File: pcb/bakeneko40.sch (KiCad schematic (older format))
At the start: 15 parts

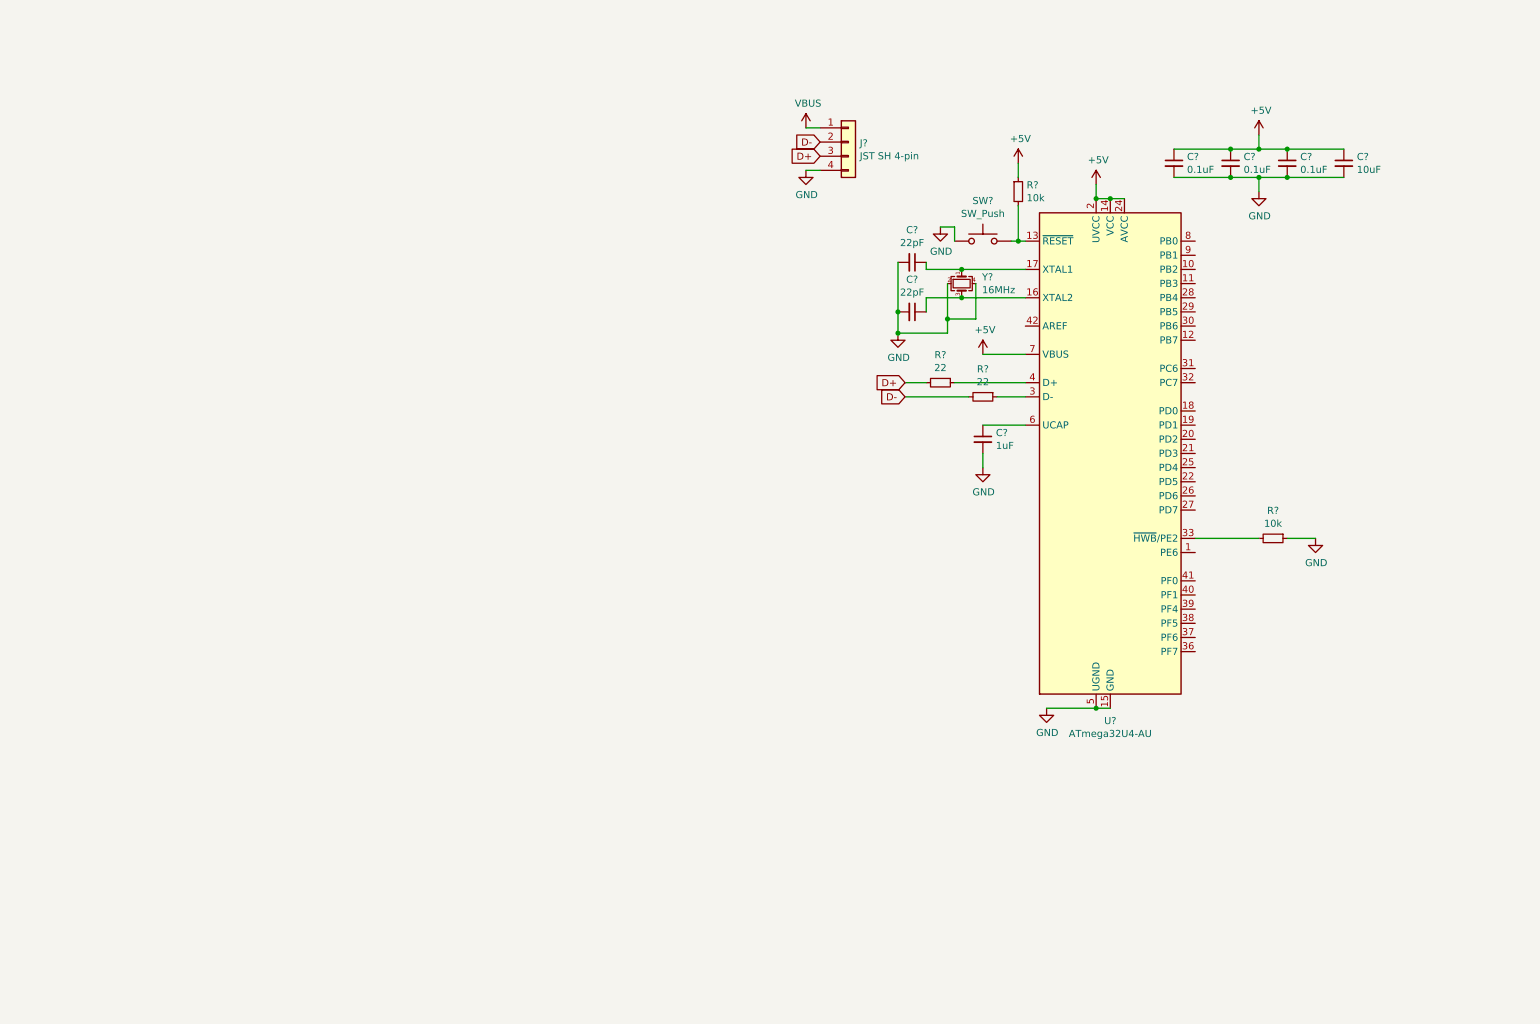
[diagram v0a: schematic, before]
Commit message: sch updates
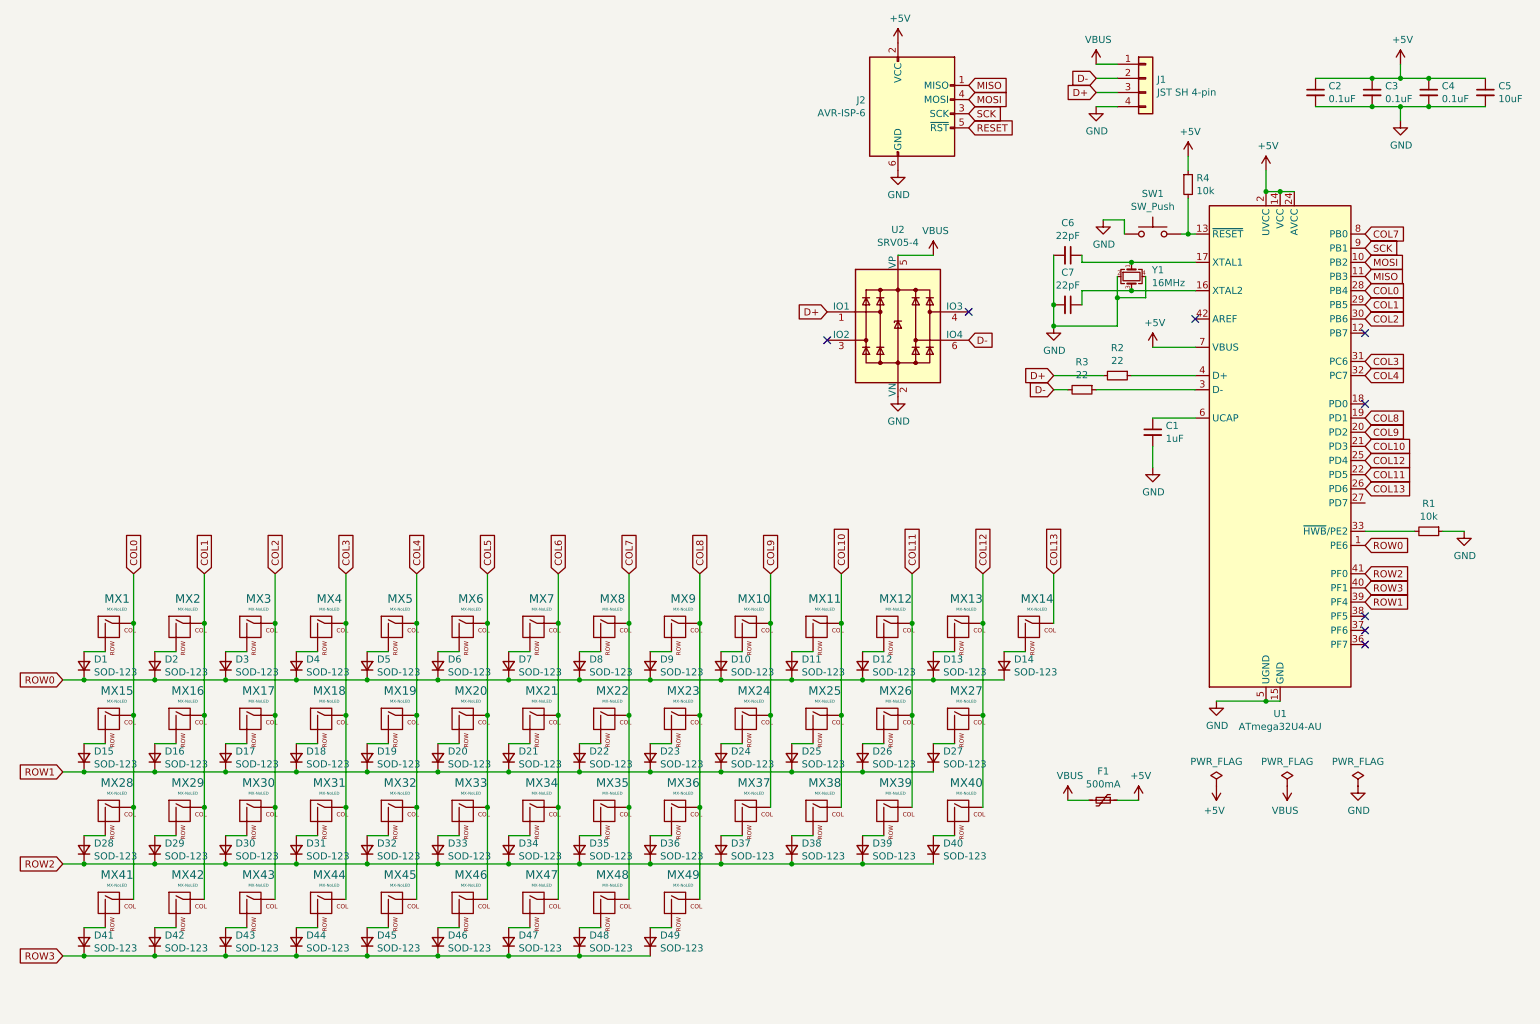
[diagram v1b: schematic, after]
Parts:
- removed C?: 1uF, symbol Device:C_Small
- removed C? (x3): 0.1uF, symbol Device:C_Small
- removed C?: 10uF, symbol Device:C_Small
- removed C? (x2): 22pF, symbol Device:C_Small
- removed J?: JST SH 4-pin, Connector_JST:JST_SH_SM04B-SRSS-TB_1x04-1MP_P1.00mm_Horizontal, symbol Connector_Generic:Conn_01x04
- removed R? (x2): 10k, symbol Device:R_Small
- removed R? (x2): 22, symbol Device:R_Small
- removed SW?: SW_Push, symbol Switch:SW_Push
- removed U?: ATmega32U4-AU, Package_QFP:TQFP-44_10x10mm_P0.8mm, symbol MCU_Microchip_ATmega:ATmega32U4-AU
- removed Y?: 16MHz, symbol Device:Crystal_GND24_Small
- added C1: 1uF, Capacitor_SMD:C_0805_2012Metric, symbol Device:C_Small
- added C2, C3, C4: 0.1uF, Capacitor_SMD:C_0805_2012Metric, symbol Device:C_Small
- added C5: 10uF, Capacitor_SMD:C_0805_2012Metric, symbol Device:C_Small
- added C6: 22pF, Capacitor_SMD:C_0805_2012Metric, symbol Device:C_Small
- added C7: 22pF, Diode_SMD:D_SOD-123, symbol Device:C_Small
- added D1, D10, D11, D12, D13, D14, D15, D16, D17, D18, D19, D2, D20, D21, D22, D23, D24, D25, D26, D27, D28, D29, D3, D30, D31, D32, D33, D34, D35, D36, D37, D38, D39, D4, D40, D41, D42, D43, D44, D45, D46, D47, D48, D49, D5, D6, D7, D8, D9: SOD-123, Diode_SMD:D_SOD-123, symbol Device:D_Small
- added F1: 500mA, Fuse:Fuse_1206_3216Metric, symbol Device:Polyfuse_Small
- added J1: JST SH 4-pin, random-keyboard-parts:JST-SR-4, symbol Connector_Generic:Conn_01x04
- added J2: AVR-ISP-6, random-keyboard-parts:Reset_Pretty-Mask, symbol Connector:AVR-ISP-6
- added MX1, MX10, MX11, MX12, MX13, MX14, MX16, MX17, MX18, MX19, MX2, MX20, MX21, MX22, MX23, MX24, MX25, MX26, MX29, MX3, MX30, MX31, MX32, MX33, MX34, MX35, MX36, MX37, MX38, MX4, MX40, MX49, MX5, MX6, MX7, MX8, MX9: MX-NoLED, MX_Only:MXOnly-1U-NoLED, symbol MX_Alps_Hybrid:MX-NoLED
- added MX15, MX39, MX41, MX43, MX46, MX48: MX-NoLED, MX_Only:MXOnly-1.25U-NoLED, symbol MX_Alps_Hybrid:MX-NoLED
- added MX27, MX28: MX-NoLED, MX_Only:MXOnly-1.75U-NoLED, symbol MX_Alps_Hybrid:MX-NoLED
- added MX42, MX47: MX-NoLED, MX_Only:MXOnly-1.5U-NoLED, symbol MX_Alps_Hybrid:MX-NoLED
- added MX44: MX-NoLED, MX_Only:MXOnly-2.25U-NoLED, symbol MX_Alps_Hybrid:MX-NoLED
- added MX45: MX-NoLED, MX_Only:MXOnly-2.75U-NoLED, symbol MX_Alps_Hybrid:MX-NoLED
- added R1, R4: 10k, Resistor_SMD:R_0805_2012Metric, symbol Device:R_Small
- added R2, R3: 22, Resistor_SMD:R_0805_2012Metric, symbol Device:R_Small
- added SW1: SW_Push, random-keyboard-parts:SKQG-1155865, symbol Switch:SW_Push
- added U1: ATmega32U4-AU, Package_QFP:TQFP-44_10x10mm_P0.8mm, symbol MCU_Microchip_ATmega:ATmega32U4-AU
- added U2: SRV05-4, Package_TO_SOT_SMD:SOT-23-6, symbol Power_Protection:SRV05-4
- added Y1: 16MHz, Crystal:Crystal_SMD_3225-4Pin_3.2x2.5mm, symbol Device:Crystal_GND24_Small
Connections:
- net +5V: now also C2.1, C3.1, C4.1, C5.1, F1.1, J2.2 (VCC), R4.1, U1.14 (VCC), U1.2 (UVCC), U1.24 (AVCC), U1.34 (VCC), U1.44 (AVCC), U1.7 (VBUS)
- net D+: now also J1.3 (Pin_3), R2.2, U2.1 (IO1)
- net D-: now also J1.2 (Pin_2), R3.2, U2.6 (IO4)
- net GND: now also C1.2, C2.2, C3.2, C4.2, C5.2, C6.2, C7.2, J1.4 (Pin_4), J2.6 (GND), R1.1, SW1.1, U1.15 (GND), U1.23 (GND), U1.35 (GND), U1.43 (GND), U1.5 (UGND), U2.2 (VN), Y1.2, Y1.4
- net VBUS: now also F1.2, J1.1 (Pin_1), U2.5 (VP)
- new net: R2.1, U1.4 (D+)
- new net: R3.1, U1.3 (D-)
- new net: C1.1, U1.6 (UCAP)
- new net: C6.1, U1.17 (XTAL1), Y1.1
- new net: C7.1, U1.16 (XTAL2), Y1.3
- new net: R4.2, SW1.2, U1.13 (~RESET)
- new net: D1.2 (A), MX1.2 (ROW)
- new net: D2.2 (A), MX2.2 (ROW)
- new net: D3.2 (A), MX3.2 (ROW)
- new net: D4.2 (A), MX4.2 (ROW)
- new net: D5.2 (A), MX5.2 (ROW)
- new net: D6.2 (A), MX6.2 (ROW)
- new net: D7.2 (A), MX7.2 (ROW)
- new net: D8.2 (A), MX8.2 (ROW)
- new net: D9.2 (A), MX9.2 (ROW)
- new net: D10.2 (A), MX10.2 (ROW)
- new net: D11.2 (A), MX11.2 (ROW)
- new net: D12.2 (A), MX12.2 (ROW)
- new net: D13.2 (A), MX13.2 (ROW)
- new net: D14.2 (A), MX14.2 (ROW)
- new net: D15.2 (A), MX15.2 (ROW)
- new net: D16.2 (A), MX16.2 (ROW)
- new net: D17.2 (A), MX17.2 (ROW)
- new net: D18.2 (A), MX18.2 (ROW)
- new net: D19.2 (A), MX19.2 (ROW)
- new net: D20.2 (A), MX20.2 (ROW)
- new net: D21.2 (A), MX21.2 (ROW)
- new net: D22.2 (A), MX22.2 (ROW)
- new net: D23.2 (A), MX23.2 (ROW)
- new net: D24.2 (A), MX24.2 (ROW)
- new net: D25.2 (A), MX25.2 (ROW)
- new net: D26.2 (A), MX26.2 (ROW)
- new net: D27.2 (A), MX27.2 (ROW)
- new net: D28.2 (A), MX28.2 (ROW)
- new net: D29.2 (A), MX29.2 (ROW)
- new net: D30.2 (A), MX30.2 (ROW)
- new net: D31.2 (A), MX31.2 (ROW)
- new net: D32.2 (A), MX32.2 (ROW)
- new net: D33.2 (A), MX33.2 (ROW)
- new net: D34.2 (A), MX34.2 (ROW)
- new net: D35.2 (A), MX35.2 (ROW)
- new net: D36.2 (A), MX36.2 (ROW)
- new net: D37.2 (A), MX37.2 (ROW)
- new net: D38.2 (A), MX38.2 (ROW)
- new net: D39.2 (A), MX39.2 (ROW)
- new net: D40.2 (A), MX40.2 (ROW)
- new net: D41.2 (A), MX41.2 (ROW)
- new net: D42.2 (A), MX42.2 (ROW)
- new net: D43.2 (A), MX43.2 (ROW)
- new net: D44.2 (A), MX44.2 (ROW)
- new net: D45.2 (A), MX45.2 (ROW)
- new net: D46.2 (A), MX46.2 (ROW)
- new net: D47.2 (A), MX47.2 (ROW)
- new net: D48.2 (A), MX48.2 (ROW)
- new net: D49.2 (A), MX49.2 (ROW)
- new net: R1.2, U1.33 (~HWB~/PE2)
- new net COL0: MX1.1 (COL), MX15.1 (COL), MX28.1 (COL), MX41.1 (COL), U1.28 (PB4)
- new net COL1: MX16.1 (COL), MX2.1 (COL), MX29.1 (COL), MX42.1 (COL), U1.29 (PB5)
- new net COL10: MX11.1 (COL), MX25.1 (COL), MX38.1 (COL), U1.21 (PD3)
- new net COL11: MX12.1 (COL), MX26.1 (COL), MX39.1 (COL), U1.22 (PD5)
- new net COL12: MX13.1 (COL), MX27.1 (COL), MX40.1 (COL), U1.25 (PD4)
- new net COL13: MX14.1 (COL), U1.26 (PD6)
- new net COL2: MX17.1 (COL), MX3.1 (COL), MX30.1 (COL), MX43.1 (COL), U1.30 (PB6)
- new net COL3: MX18.1 (COL), MX31.1 (COL), MX4.1 (COL), MX44.1 (COL), U1.31 (PC6)
- new net COL4: MX19.1 (COL), MX32.1 (COL), MX45.1 (COL), MX5.1 (COL), U1.32 (PC7)
- new net COL5: MX20.1 (COL), MX33.1 (COL), MX46.1 (COL), MX6.1 (COL)
- new net COL6: MX21.1 (COL), MX34.1 (COL), MX47.1 (COL), MX7.1 (COL)
- new net COL7: MX22.1 (COL), MX35.1 (COL), MX48.1 (COL), MX8.1 (COL), U1.8 (PB0)
- new net COL8: MX23.1 (COL), MX36.1 (COL), MX49.1 (COL), MX9.1 (COL), U1.19 (PD1)
- new net COL9: MX10.1 (COL), MX24.1 (COL), MX37.1 (COL), U1.20 (PD2)
- new net MISO: J2.1 (MISO), U1.11 (PB3)
- new net MOSI: J2.4 (MOSI), U1.10 (PB2)
- new net RESET: J2.5 (~RST)
- new net ROW0: D1.1 (K), D10.1 (K), D11.1 (K), D12.1 (K), D13.1 (K), D14.1 (K), D2.1 (K), D3.1 (K), D4.1 (K), D5.1 (K), D6.1 (K), D7.1 (K), D8.1 (K), D9.1 (K), U1.1 (PE6)
- new net ROW1: D15.1 (K), D16.1 (K), D17.1 (K), D18.1 (K), D19.1 (K), D20.1 (K), D21.1 (K), D22.1 (K), D23.1 (K), D24.1 (K), D25.1 (K), D26.1 (K), D27.1 (K), U1.39 (PF4)
- new net ROW2: D28.1 (K), D29.1 (K), D30.1 (K), D31.1 (K), D32.1 (K), D33.1 (K), D34.1 (K), D35.1 (K), D36.1 (K), D37.1 (K), D38.1 (K), D39.1 (K), D40.1 (K), U1.41 (PF0)
- new net ROW3: D41.1 (K), D42.1 (K), D43.1 (K), D44.1 (K), D45.1 (K), D46.1 (K), D47.1 (K), D48.1 (K), D49.1 (K), U1.40 (PF1)
- new net SCK: J2.3 (SCK), U1.9 (PB1)
- no-connect marks 0 -> 8

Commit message: pcb routing
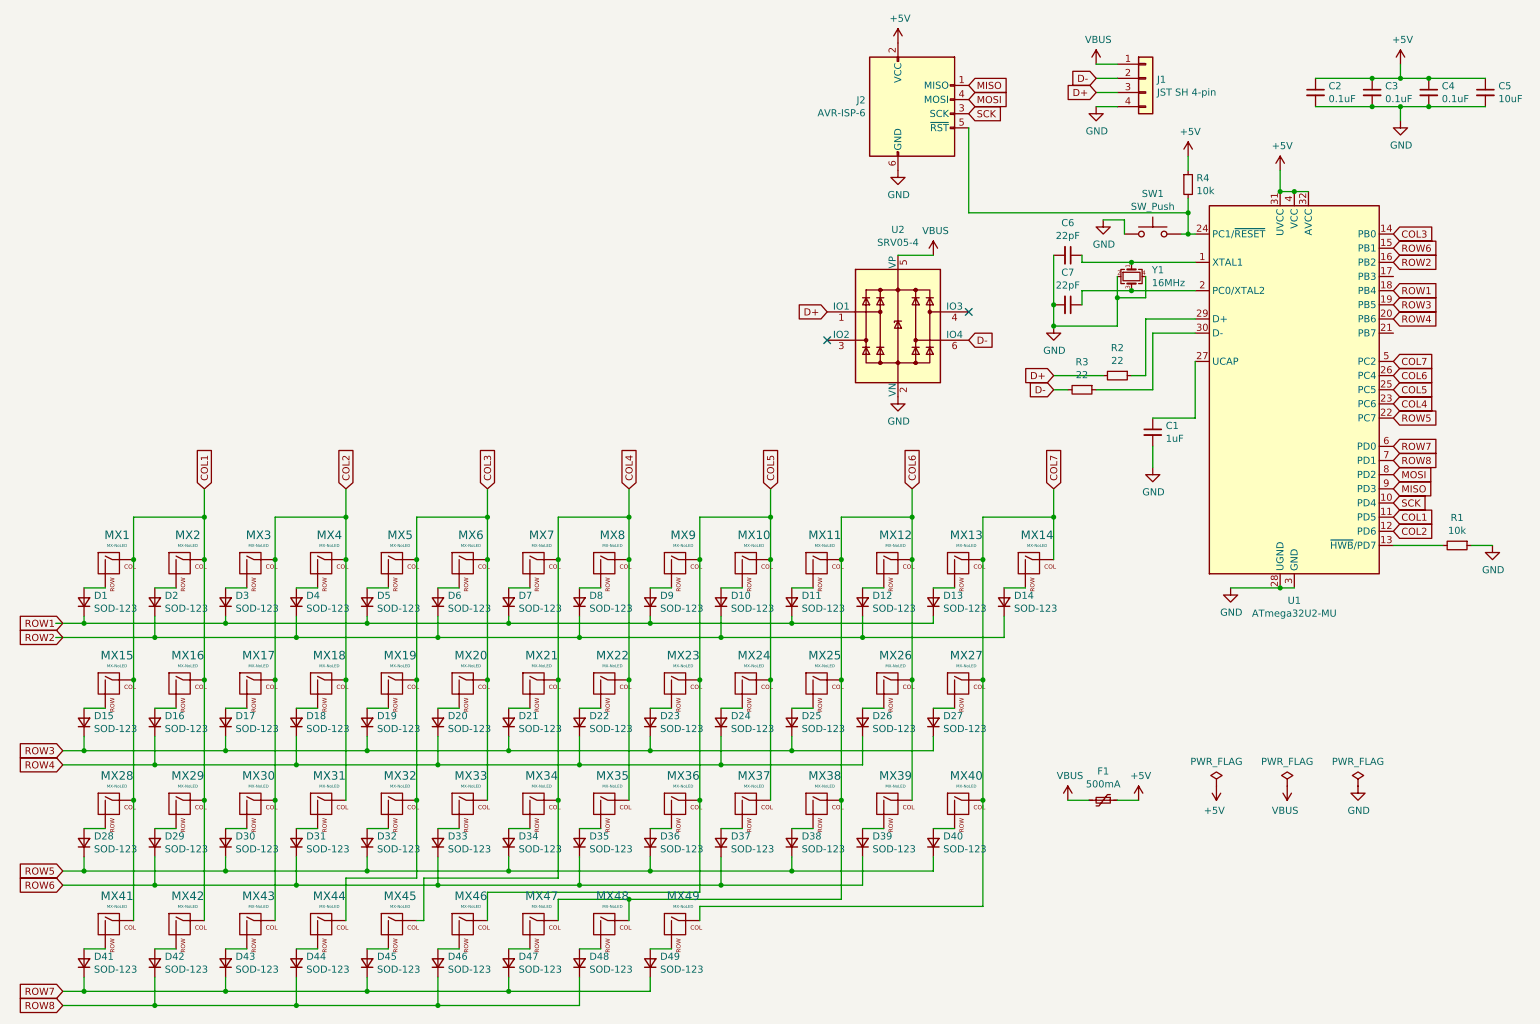
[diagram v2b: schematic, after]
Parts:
- removed U1: ATmega32U4-AU, Package_QFP:TQFP-44_10x10mm_P0.8mm, symbol MCU_Microchip_ATmega:ATmega32U4-AU
- added U1: ATmega32U2-MU, Package_DFN_QFN:QFN-32-1EP_5x5mm_P0.5mm_EP3.1x3.1mm, symbol MCU_Microchip_ATmega:ATmega32U2-MU
- C7: footprint Diode_SMD:D_SOD-123 -> Capacitor_SMD:C_0805_2012Metric
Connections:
- net COL0 is gone; now on net COL1: MX1.1 (COL), MX15.1 (COL), MX28.1 (COL), MX41.1 (COL)
- net COL10 is gone; now on net COL6: MX11.1 (COL), MX25.1 (COL), MX38.1 (COL)
- net COL11 is gone; now on net COL6: MX12.1 (COL), MX26.1 (COL), MX39.1 (COL)
- net COL12 is gone; now on net COL7: MX13.1 (COL), MX27.1 (COL), MX40.1 (COL)
- net COL13 is gone; now on net COL7: MX14.1 (COL)
- net COL9 is gone; now on net COL5: MX10.1 (COL), MX24.1 (COL), MX37.1 (COL)
- net RESET is gone; now on an unnamed net: J2.5 (~RST)
- net +5V: now also U1.31 (UVCC), U1.32 (AVCC), U1.4 (VCC)
- net COL1: now also U1.11 (PD5)
- net COL2: now also MX18.1 (COL), MX31.1 (COL), MX4.1 (COL), U1.12 (PD6)
- net COL3: now also MX19.1 (COL), MX20.1 (COL), MX32.1 (COL), MX33.1 (COL), MX5.1 (COL), MX6.1 (COL), U1.14 (PB0); no longer MX18.1 (COL), MX31.1 (COL), MX4.1 (COL)
- net COL4: now also MX21.1 (COL), MX22.1 (COL), MX34.1 (COL), MX35.1 (COL), MX7.1 (COL), MX8.1 (COL), U1.23 (PC6); no longer MX19.1 (COL), MX32.1 (COL), MX5.1 (COL)
- net COL5: now also MX23.1 (COL), MX36.1 (COL), MX9.1 (COL), U1.25 (PC5); no longer MX20.1 (COL), MX33.1 (COL), MX6.1 (COL)
- net COL6: now also MX48.1 (COL), U1.26 (PC4); no longer MX21.1 (COL), MX34.1 (COL), MX7.1 (COL)
- net COL7: now also MX49.1 (COL), U1.5 (PC2); no longer MX22.1 (COL), MX35.1 (COL), MX48.1 (COL), MX8.1 (COL)
- net GND: now also U1.28 (UGND), U1.3 (GND), U1.33 (GND)
- net MISO: now also U1.9 (PD3)
- net MOSI: now also U1.8 (PD2)
- net ROW1: now also D1.1 (K), D11.1 (K), D13.1 (K), D3.1 (K), D5.1 (K), D7.1 (K), D9.1 (K), U1.18 (PB4); no longer D15.1 (K), D16.1 (K), D17.1 (K), D18.1 (K), D19.1 (K), D20.1 (K), D21.1 (K), D22.1 (K), D23.1 (K), D24.1 (K), D25.1 (K), D26.1 (K), D27.1 (K)
- net ROW2: now also D10.1 (K), D12.1 (K), D14.1 (K), D2.1 (K), D4.1 (K), D6.1 (K), D8.1 (K), U1.16 (PB2); no longer D28.1 (K), D29.1 (K), D30.1 (K), D31.1 (K), D32.1 (K), D33.1 (K), D34.1 (K), D35.1 (K), D36.1 (K), D37.1 (K), D38.1 (K), D39.1 (K), D40.1 (K)
- net ROW3: now also D15.1 (K), D17.1 (K), D19.1 (K), D21.1 (K), D23.1 (K), D25.1 (K), D27.1 (K), U1.19 (PB5); no longer D41.1 (K), D42.1 (K), D43.1 (K), D44.1 (K), D45.1 (K), D46.1 (K), D47.1 (K), D48.1 (K), D49.1 (K)
- net SCK: now also U1.10 (PD4)
- net at R2.1: now also U1.29 (D+)
- net at R3.1: now also U1.30 (D-)
- net at C1.1: now also U1.27 (UCAP)
- net at C6.1, Y1.1: now also U1.1 (XTAL1)
- net at C7.1, Y1.3: now also U1.2 (PC0/XTAL2)
- net at R4.2, SW1.2: now also U1.24 (PC1/~RESET)
- net at R1.2: now also U1.13 (~HWB~/PD7)
- removed net COL8: MX23.1 (COL), MX36.1 (COL), MX49.1 (COL), MX9.1 (COL)
- removed net ROW0: D1.1 (K), D10.1 (K), D11.1 (K), D12.1 (K), D13.1 (K), D14.1 (K), D2.1 (K), D3.1 (K), D4.1 (K), D5.1 (K), D6.1 (K), D7.1 (K), D8.1 (K), D9.1 (K)
- new net ROW4: D16.1 (K), D18.1 (K), D20.1 (K), D22.1 (K), D24.1 (K), D26.1 (K), U1.20 (PB6)
- new net ROW5: D28.1 (K), D30.1 (K), D32.1 (K), D34.1 (K), D36.1 (K), D38.1 (K), D40.1 (K), U1.22 (PC7)
- new net ROW6: D29.1 (K), D31.1 (K), D33.1 (K), D35.1 (K), D37.1 (K), D39.1 (K), U1.15 (PB1)
- new net ROW7: D41.1 (K), D43.1 (K), D45.1 (K), D47.1 (K), D49.1 (K), U1.6 (PD0)
- new net ROW8: D42.1 (K), D44.1 (K), D46.1 (K), D48.1 (K), U1.7 (PD1)
- no-connect marks 8 -> 2
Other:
- moved on the sheet: D1, D10, D11, D12, D13, D14, D15, D16, D17, D18, D19, D2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
